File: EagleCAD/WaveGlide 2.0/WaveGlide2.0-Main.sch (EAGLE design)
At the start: 8 parts, among them IC1 TPS77033, K1 AQY21SOP, K2 MS-20-310-HN, U1 ATMEGA328P_TQFP, U2 BMP180, U3 MPXV7002, X1 22-23-2111

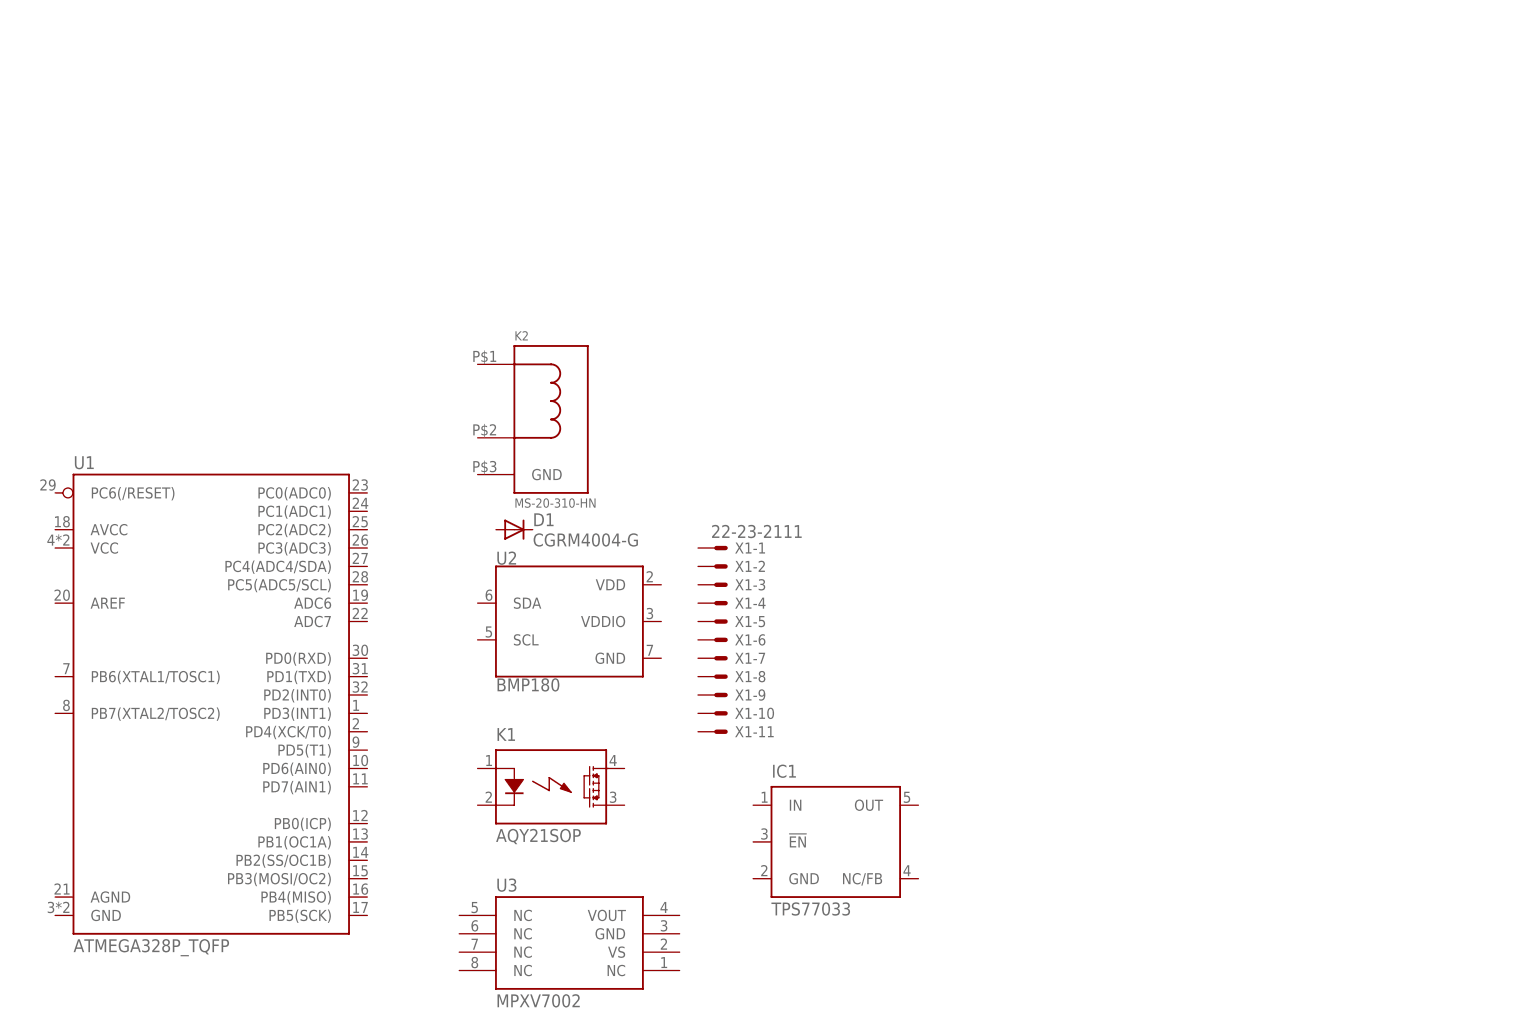
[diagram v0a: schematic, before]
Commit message: Updated Schematic
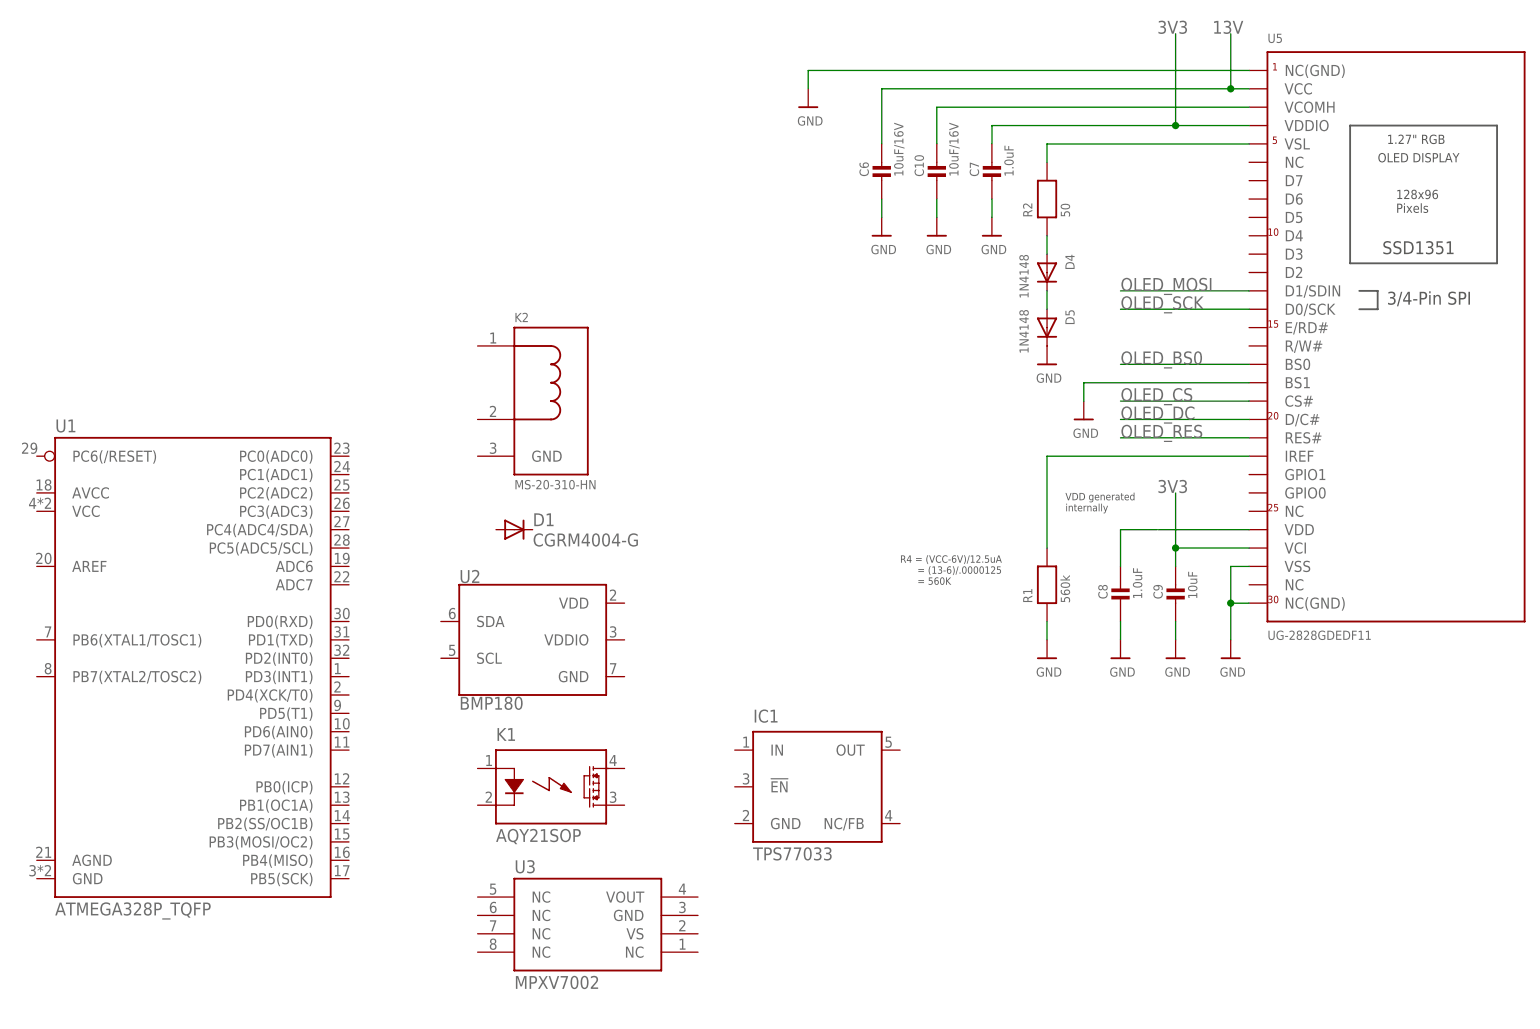
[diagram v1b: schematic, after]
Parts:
- removed X1: 22-23-2111, con-molex:22-23-2111
- added C10, C6: 10uF/16V, microbuilder:CAP_CERAMIC_0805MP
- added C7, C8: 1.0uF, microbuilder:CAP_CERAMIC_0805MP
- added C9: 10uF, microbuilder:CAP_CERAMIC_0805MP
- added D4, D5: 1N4148, microbuilder:DIODESOD-323
- added R1: 560k, microbuilder:RESISTOR_0805MP
- added R2: 50, microbuilder:RESISTOR_0805MP
- added U5: UG-2828GDEDF11, microbuilder:DISP_OLED_UG-2896GDEAF11TOP
- IC1: device texas:TPS77033 -> CustomParts:TPS77033
- U1: device SparkFun-IC-Microcontroller:ATMEGA328P_TQFP -> CustomParts:ATMEGA328P_TQFP
- U2: device SparkFun-Sensors:BMP180 -> CustomParts:BMP180
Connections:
- new net 13V: C6.1, U5.VCC
- new net 3V3: C7.1, C9.1, U5.VCI, U5.VDDIO
- new net GND: C10.2, C6.2, C7.2, C8.2, C9.2, D5.C, R1.1, U5.BS1, U5.NC(GND)@1, U5.NC(GND)@2, U5.VSS
- new net N$2: D4.A, R2.1
- new net N$3: C10.1, U5.VCOMH
- new net N$4: U5.VDD
- new net N$5: D4.C, D5.A
- new net N$6: C8.1
- new net N$7: R1.2, U5.IREF
- new net N$8: R2.2, U5.VSL
- new net OLED_BS0: U5.BS0
- new net OLED_CS: U5.CS#
- new net OLED_DC: U5.D/C#
- new net OLED_MOSI: U5.D1/SDIN
- new net OLED_RES: U5.RES#
- new net OLED_SCK: U5.D0/SCK
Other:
- note added: "R4 = (VCC-6V)/12.5uA = (13-6)/.0000125 = 560K"
- note added: "VDD generated internally"
- moved on the sheet: IC1, K2, U1, U2, U3

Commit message: Start generating schematic
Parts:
- removed IC1: TPS77033, CustomParts:TPS77033
- removed K1: AQY21SOP, relay:AQY21SOP
- added C1: 0.1uF, microbuilder:CAP_CERAMIC_0805MP
- added CN3: 0, microbuilder:USBMICRO_20329
- added D6: 3.6v, microbuilder:DIODESOD-323
- added D7: 3.6V, microbuilder:DIODESOD-323
- added JP1: 0, pinhead:PINHD-2X3
- added Q2: reset, microbuilder:SWITCH_TACT_SMT4.6X2.8
- added R10: 1.5K (0603), microbuilder:RESISTOR_0603_NOOUT
- added R12: 10K, microbuilder:RESISTOR0805_NOOUTLINE
- added R14: 10k, resistor:R-US_R0603
- added R8, R9: 68 (0603), microbuilder:RESISTOR_0603_NOOUT
- added Y2: 12MHz, SparkFun:RESONATORSMD
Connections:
- net 13V renamed SYS_13V
- net N$3 renamed OLED_VCOMH
- net N$7 renamed OLED_IREF
- net N$8 renamed OLED_VSL
- removed net 3V3: C7.1, C9.1, U5.VCI, U5.VDDIO
- removed net N$4: U5.VDD
- removed net N$6: C8.1
- removed net OLED_BS0: U5.BS0
- removed net OLED_CS: U5.CS#
- removed net OLED_DC: U5.D/C#
- removed net OLED_MOSI: U5.D1/SDIN
- removed net OLED_RES: U5.RES#
- removed net OLED_SCK: U5.D0/SCK
- new net BMP180_3V3: U2.VDD, U2.VDDIO
- new net D+1: CN3.D+, D6.C, R9.1
- new net D-1: CN3.D-, D7.C, R10.1, R8.1
- new net MCU_AREF: C1.1, U1.AREF
- new net MCU_I2C_SCL: U1.PC5(ADC5/SCL), U2.SCL
- new net MCU_I2C_SDA: U1.PC4(ADC4/SDA), U2.SDA
- new net MCU_OLED_CS: R14.1, U1.PB2(SS/OC1B), U5.CS#
- new net MCU_OLED_DC: U1.PB0(ICP), U5.D/C#
- new net MCU_OLED_RES: U1.PB1(OC1A), U5.RES#
- new net MCU_PROG/OLED_MOSI: JP1.4, U1.PB3(MOSI/OC2), U5.D1/SDIN
- new net MCU_PROG/OLED_SCK: JP1.3, U1.PB5(SCK), U5.D0/SCK
- new net MCU_PROG_MISO: JP1.1, U1.PB4(MISO)
- new net MCU_RESET: JP1.5, Q2.P, Q2.P1, R12.1, U1.PC6(/RESET)
- new net MPXV_5V: U3.VS
- new net MPXV_VS: U1.PC3(ADC3), U3.VOUT
- new net N$10: U1.PB7(XTAL2/TOSC2), Y2.3
- new net N$9: U1.PB6(XTAL1/TOSC1), Y2.1
- new net OLED_VDD: C8.1, U5.VDD
- new net SOLENOID_12V: D1.C, K2.VS
- new net SYS_3V3: C7.1, C9.1, R10.2, R12.2, R14.2, U1.AVCC, U1.VCC, U5.VCI, U5.VDDIO
- new net USB_D+: R9.2, U1.PD2(INT0)
- new net USB_D-: R8.2, U1.PD7(AIN1)
- new net VBUS: CN3.VBUS
- net GND: now also C1.2, CN3.GND, D1.A, D6.A, D7.A, JP1.6, K2.GND, K2.VR, Q2.S, Q2.S1, U1.AGND, U1.GND, U2.GND, U3.GND, U5.BS0, U5.D3, U5.D4, U5.D5, U5.D6, U5.D7, U5.E/RD#, U5.R/W#, Y2.2
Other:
- moved on the sheet: C10, C6, C7, C8, C9, D1, D4, D5, K2, R1, R2, U1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
